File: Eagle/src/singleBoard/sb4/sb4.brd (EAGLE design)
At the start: 82.5 x 97.3 mm, 49 parts, among them U1 GY-521MPU6050

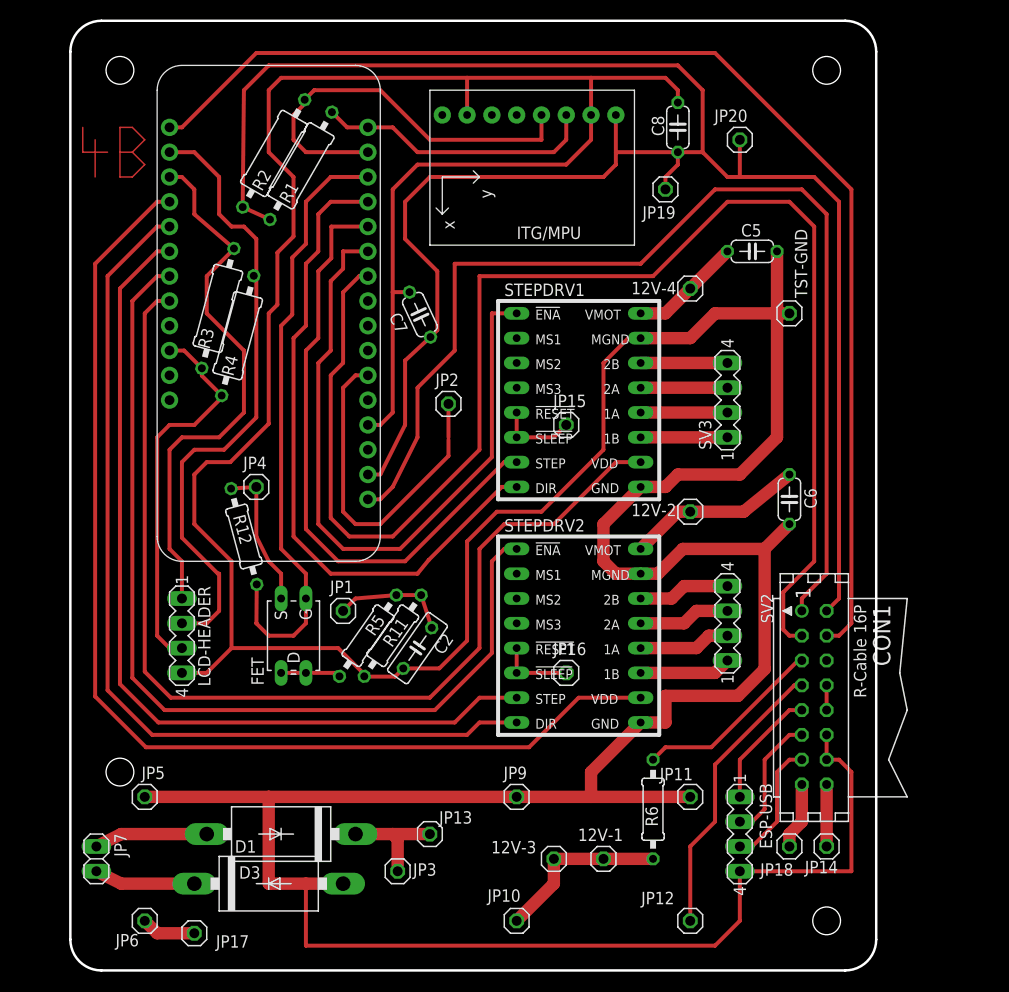
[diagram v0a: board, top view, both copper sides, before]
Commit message: minor updates
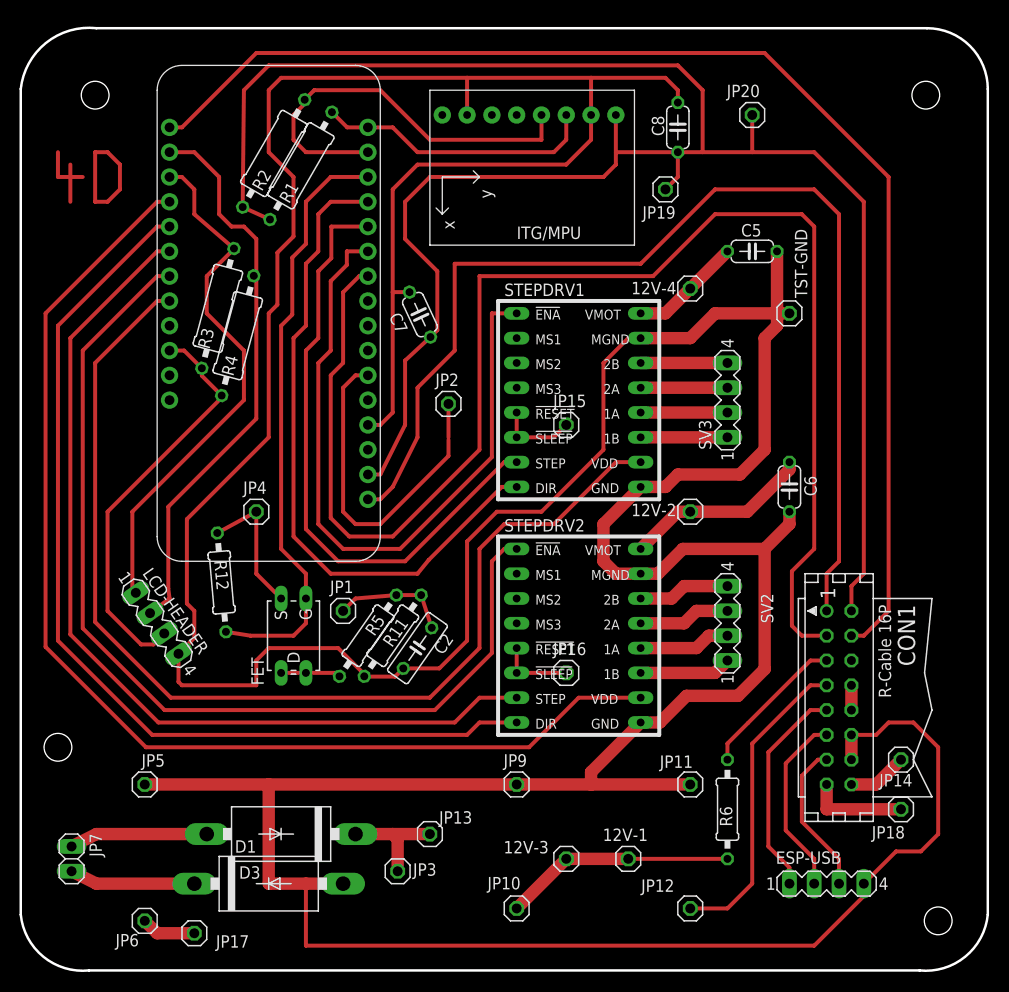
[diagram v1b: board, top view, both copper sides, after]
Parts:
- moved JP18 12.0 mm to (85.1, 16.5)
- moved JP14 11.7 mm to (85.1, 21.6)
- moved ESP-USB 10.2 mm to (77.5, 8.89), turned to 0 degrees
- moved R6 7.62 mm to (67.3, 16.5)
- moved R12 5.23 mm to (15.5, 39.8), turned to 275 degrees
- moved LCD-HEADER 2.84 mm to (8.89, 35.6), turned to 305 degrees
- moved JP20 2.84 mm to (69.8, 87.6)
- moved JP7 2.54 mm to (0.13, 11.4)
- moved 12V-1 2.54 mm to (57.1, 11.4)
- moved JP4 2.54 mm to (19.1, 47.0)
- moved CON1 2.54 mm to (78.7, 27.9)
- moved C6 1.27 mm to (73.7, 49.5)
- moved JP10 1.27 mm to (45.7, 6.35)
- moved JP11 1.27 mm to (63.5, 19.1)
- moved JP12 1.27 mm to (63.5, 6.35)
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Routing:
- net N$33: track 522.2 -> 540.7 mm
- net N$55: track 12.3 -> 22.1 mm
- net N$35: track 64.1 -> 58.2 mm
- net N$22: track 13.0 -> 18.9 mm
- net N$42: track 18.1 -> 23.7 mm
- net N$28: track 126.3 -> 131.4 mm
- net N$36: track 114.7 -> 118.9 mm
- net N$34: track 90.5 -> 94.7 mm
- net N$37: track 96.6 -> 100.8 mm
- net N$29: track 95.2 -> 99.4 mm
- net N$1: track 107.6 -> 111.8 mm
- net N$2: track 19.4 -> 15.3 mm
- net N$38: track 6.88 -> 10.2 mm
- net N$23: track 13.0 -> 15.9 mm
- net USB: track 39.6 -> 42.3 mm
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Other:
- board size 82.5 x 97.3 mm -> 99.1 x 96.6 mm
